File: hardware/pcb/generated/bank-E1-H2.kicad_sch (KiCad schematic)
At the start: 34 parts, among them U10 SK9822-EC20, U11 SK9822-EC20, U12 SK9822-EC20, U13 SK9822-EC20, U14 SK9822-EC20, U15 SK9822-EC20, U16 SK9822-EC20, U17 SK9822-EC20, U2 TCA9554DWR

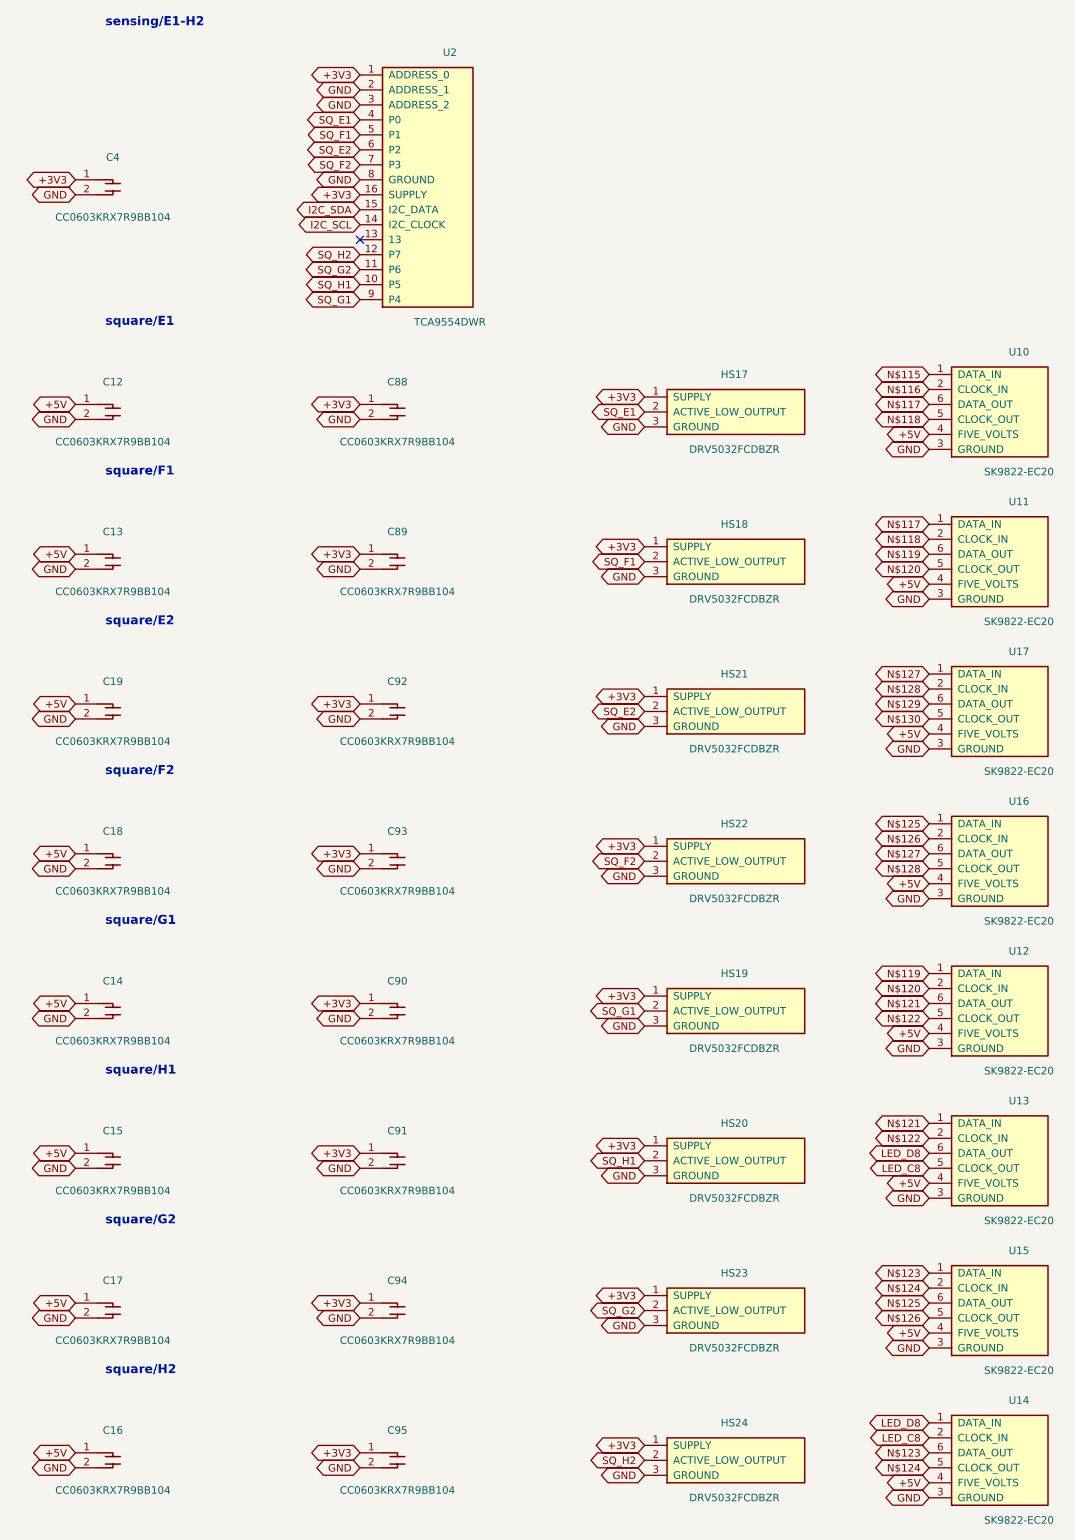
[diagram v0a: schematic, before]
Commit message: chore(pcb): regenerate KiCad, SPICE and review output
Generated by `just pcb` from the committed definition; not hand-edited.
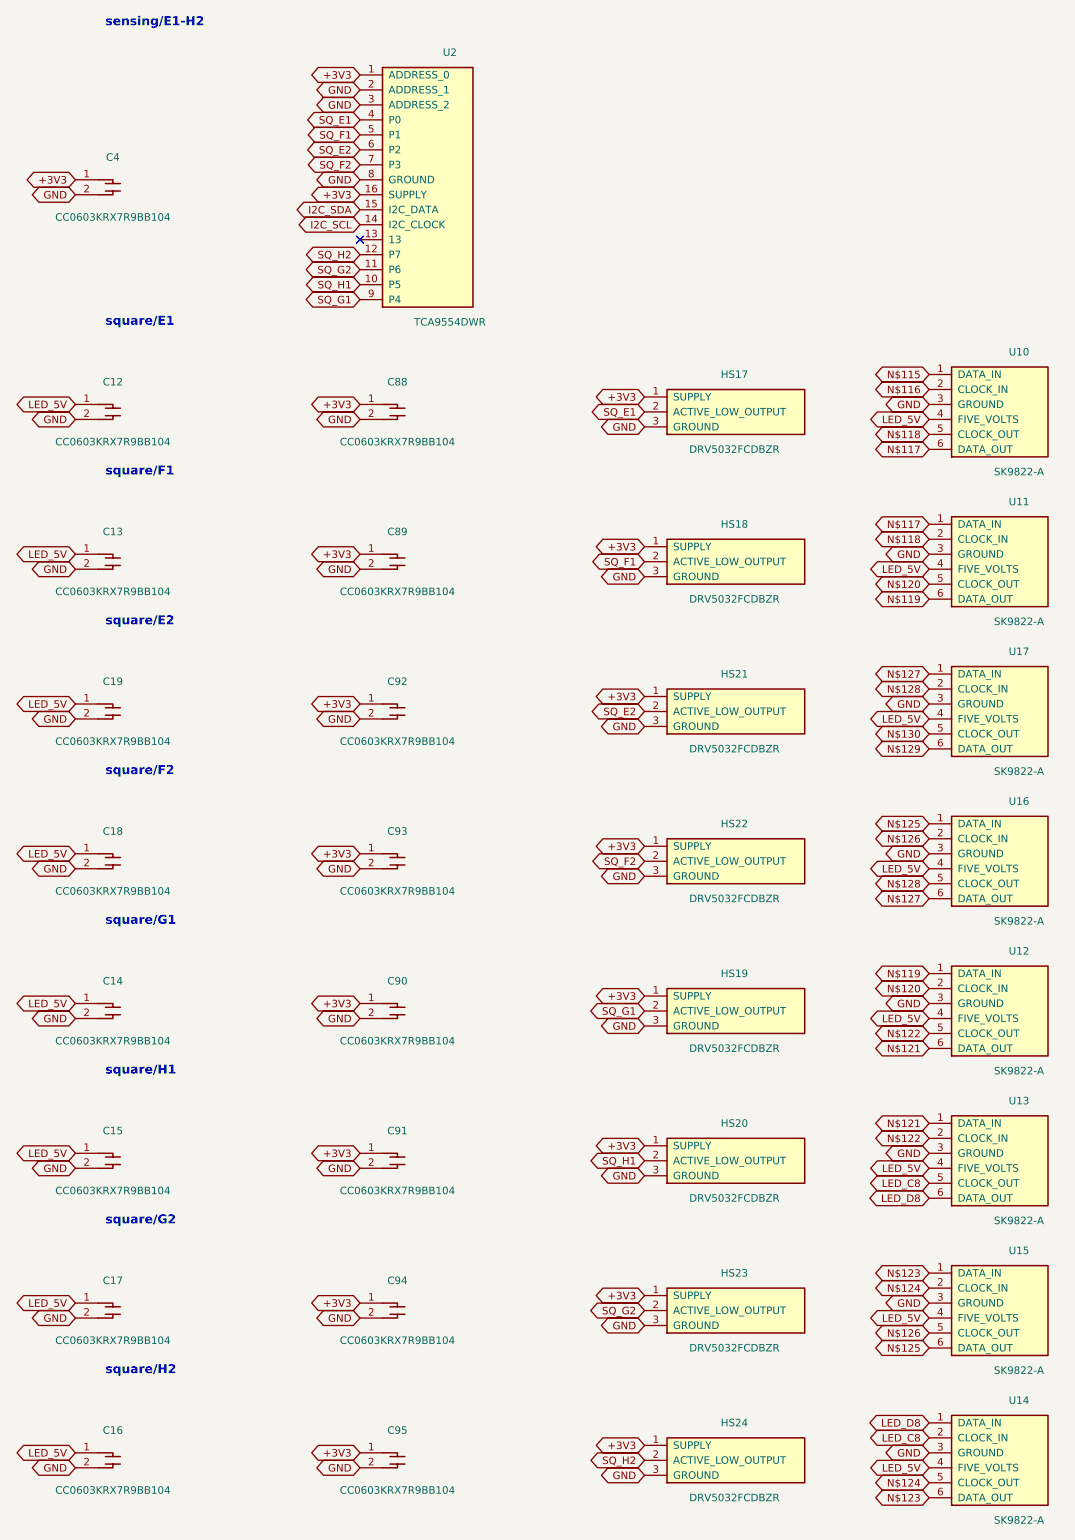
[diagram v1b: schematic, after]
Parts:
- U10, U11, U12, U13, U14, U15, U16, U17: value SK9822-EC20 -> SK9822-A
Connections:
- net +5V renamed LED_5V
